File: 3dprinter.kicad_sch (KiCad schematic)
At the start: 35 parts, among them J1 6P IDC CONNECTOR, J17 Conn_01x02, J2 USB_B, SW1 SW_Push, U1 ATmega2560-16A, U2 CH340G, U3 LM78M05_TO252, Y1 16MHZ, Y2 12MHZ

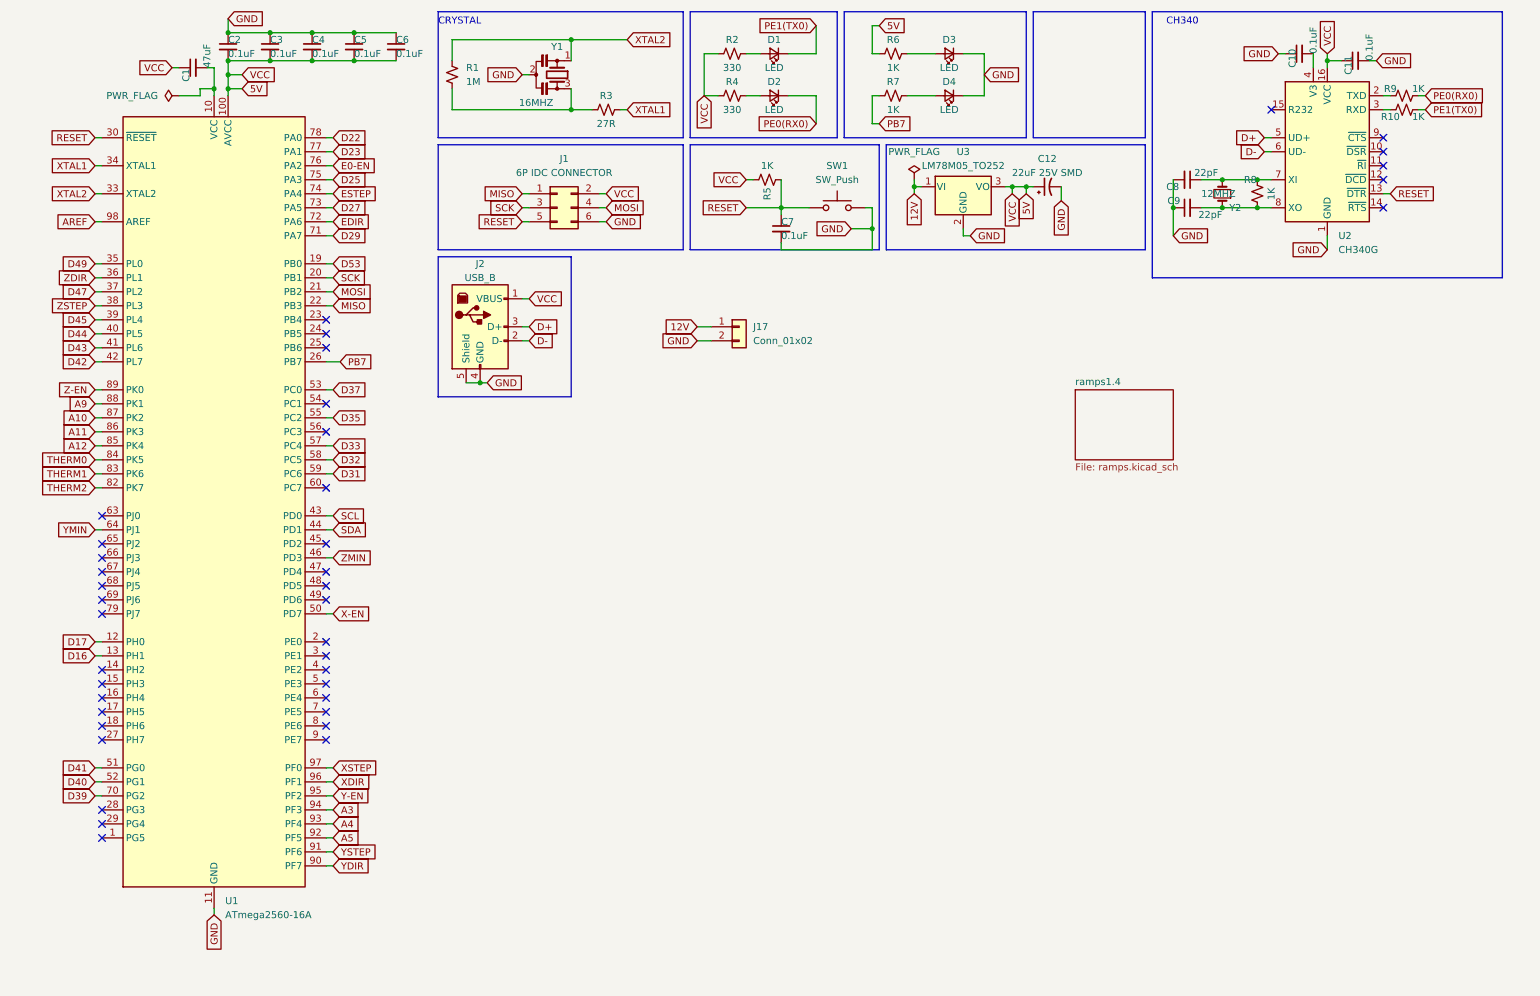
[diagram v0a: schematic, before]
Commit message: Schematic_ok
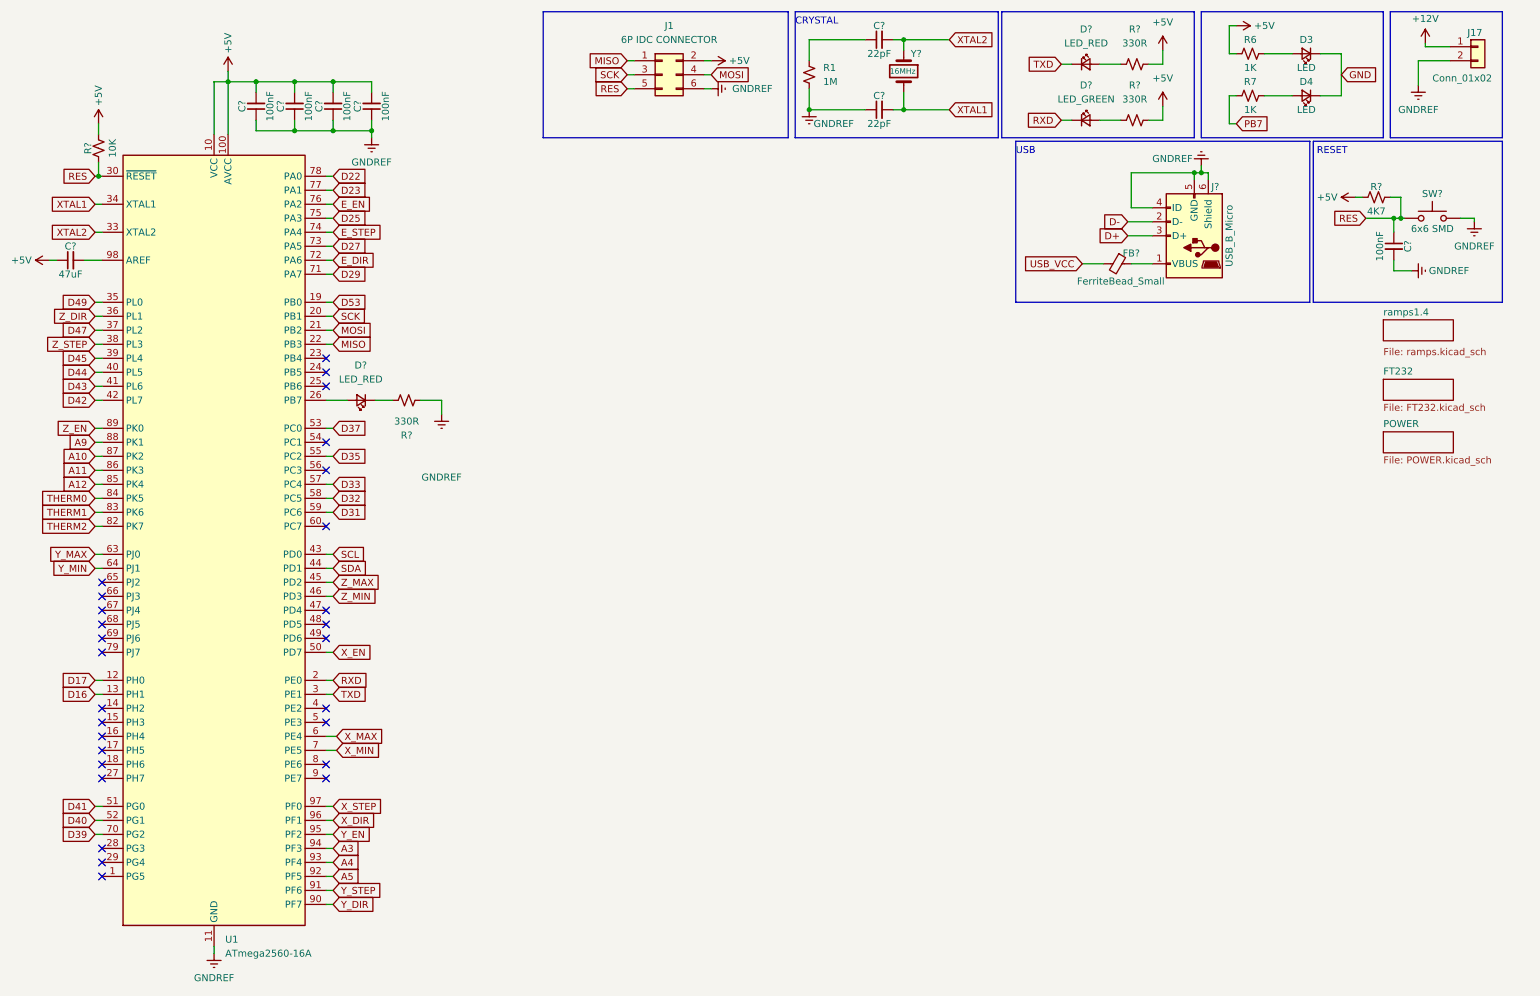
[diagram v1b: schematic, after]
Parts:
- removed C1: 47uF, Capacitor_SMD:C_0805_2012Metric, symbol Device:C_Small
- removed C10, C11, C2, C3, C4, C5, C6, C7: 0.1uF, Capacitor_SMD:C_0805_2012Metric, symbol Device:C_Small
- removed C12: 22uF 25V SMD, Capacitor_SMD:CP_Elec_6.3x7.7, symbol Device:C_Polarized_Small_US
- removed C8, C9: 22pF, Capacitor_SMD:C_0805_2012Metric, symbol Device:C_Small
- removed D1, D2: LED, LED_SMD:LED_0805_2012Metric, symbol Device:LED_Small
- removed J2: USB_B, Connector_USB:USB_B_Lumberg_2411_02_Horizontal, symbol Connector:USB_B
- removed R10, R8, R9: 1K, Resistor_SMD:R_0805_2012Metric, symbol Device:R_Small_US
- removed R2, R4: 330, Resistor_SMD:R_0805_2012Metric, symbol Device:R_Small_US
- removed R3: 27R, Resistor_SMD:R_0805_2012Metric, symbol Device:R_Small_US
- removed R5: 1K, Resistor_SMD:R_0805_2012Metric_Pad1.20x1.40mm_HandSolder, symbol Device:R_Small_US
- removed SW1: SW_Push, Button_Switch_SMD:SW_Push_1P1T_NO_6x6mm_H9.5mm, symbol Switch:SW_Push
- removed U2: CH340G, Package_SO:SOIC-16_3.9x9.9mm_P1.27mm, symbol Interface_USB:CH340G
- removed U3: LM78M05_TO252, Package_TO_SOT_SMD:TO-252-2, symbol Regulator_Linear:LM78M05_TO252
- removed Y1: 16MHZ, Crystal:Crystal_SMD_HC49-SD, symbol Device:Resonator_Small
- removed Y2: 12MHZ, Crystal:Crystal_SMD_HC49-SD, symbol Device:Crystal_Small
- added C?: 47uF, Capacitor_SMD:C_0805_2012Metric_Pad1.18x1.45mm_HandSolder, symbol Device:C_Small
- added C? (x4): 100nF, Capacitor_SMD:C_0805_2012Metric_Pad1.18x1.45mm_HandSolder, symbol Device:C_Small
- added C?: 100nF, Capacitor_SMD:C_0805_2012Metric, symbol Device:C_Small
- added C? (x2): 22pF, Capacitor_SMD:C_0805_2012Metric_Pad1.18x1.45mm_HandSolder, symbol Device:C_Small
- added D? (x2): LED_RED, LED_SMD:LED_0805_2012Metric_Pad1.15x1.40mm_HandSolder, symbol Device:LED_Small
- added D?: LED_GREEN, LED_SMD:LED_0805_2012Metric_Pad1.15x1.40mm_HandSolder, symbol Device:LED_Small
- added FB?: FerriteBead_Small, Capacitor_SMD:C_1206_3216Metric, symbol Device:FerriteBead_Small
- added J?: USB_B_Micro, Connector_USB:USB_Micro-B_GCT_USB3076-30-A, symbol Connector:USB_B_Micro
- added R?: 10K, Resistor_SMD:R_0805_2012Metric_Pad1.20x1.40mm_HandSolder, symbol Device:R_Small_US
- added R? (x3): 330R, Resistor_SMD:R_0805_2012Metric_Pad1.20x1.40mm_HandSolder, symbol Device:R_Small_US
- added R?: 4K7, Resistor_SMD:R_0805_2012Metric, symbol Device:R_Small_US
- added SW?: 6x6 SMD, Button_Switch_SMD:SW_Push_1P1T_NO_6x6mm_H9.5mm, symbol Switch:SW_Push
- added Y?: 16MHz, Crystal:Crystal_SMD_HC49-SD, symbol Device:Crystal
- J1: footprint Connector_PinHeader_2.54mm:PinHeader_2x03_P2.54mm_Vertical -> Connector_PinHeader_1.00mm:PinHeader_2x03_P1.00mm_Vertical
- J17: footprint TerminalBlock_Phoenix:TerminalBlock_Phoenix_MKDS-1,5-2-5.08_1x02_P5.08mm_Horizontal -> Connector_Phoenix_MSTB:PhoenixContact_MSTBVA_2,5_2-G-5,08_1x02_P5.08mm_Vertical
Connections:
- net 5V is gone; now on net +5V: J1.2 (Pin_2), R6.1, U1.100 (AVCC)
- net D+: now also J?.3 (D+)
- net D-: now also J?.2 (D-)
- net GND: no longer J1.6 (Pin_6), J17.2 (Pin_2), U1.11 (GND), U1.32 (GND), U1.62 (GND), U1.81 (GND), U1.99 (GND)
- net PB7: no longer U1.26 (PB7)
- net XTAL1: now also C?.2, Y?.2
- net XTAL2: now also C?.2, Y?.1; no longer R1.1
- net GNDREF: now reaches R1.2
- net GNDREF: now also J1.6 (Pin_6), J17.2 (Pin_2), U1.11 (GND), U1.32 (GND), U1.62 (GND), U1.81 (GND), U1.99 (GND), C?.1, C?.1, C?.1, C?.1, C?.1, C?.2, J?.4 (ID), J?.5 (GND), J?.6 (Shield), R?.1, SW?.2
- net +5V: now reaches U1.10 (VCC), U1.31 (VCC), U1.61 (VCC), U1.80 (VCC)
- net +5V: now also C?.1, C?.2, C?.2, C?.2, C?.2, R?.1, R?.2, R?.2, R?.2
- net RXD: now reaches U1.2 (PE0)
- net RXD: now also D?.1 (K)
- net TXD: now reaches U1.3 (PE1)
- net TXD: now also D?.1 (K)
- net Z_MAX: now reaches U1.45 (PD2)
- net X_MAX: now reaches U1.6 (PE4)
- net Y_MAX: now reaches U1.63 (PJ0)
- net X_MIN: now reaches U1.7 (PE5)
- net 12V renamed +12V
- net AREF: no longer names the net of U1.98 (AREF)
- net AREF: now also C?.2
- net E0-EN renamed E_EN
- net EDIR renamed E_DIR
- net ESTEP renamed E_STEP
- net RESET renamed RES
- net RES: now also C?.1, R?.1, R?.2, SW?.1
- net X-EN renamed X_EN
- net XDIR renamed X_DIR
- net XSTEP renamed X_STEP
- net Y-EN renamed Y_EN
- net YDIR renamed Y_DIR
- net YMIN renamed Y_MIN
- net YSTEP renamed Y_STEP
- net Z-EN renamed Z_EN
- net ZDIR renamed Z_DIR
- net ZMIN renamed Z_MIN
- net ZSTEP renamed Z_STEP
- new net: D?.2 (A), R?.1 (x2)
- new net: C?.1, R1.1
- new net: D?.2 (A), U1.26 (PB7)
- new net: D?.1 (K), R?.2
- new net: FB?.1, J?.1 (VBUS)
- new net USB_VCC: FB?.2
- no-connect marks 40 -> 28
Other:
- added sheet FT232 (FT232.kicad_sch)
- added sheet POWER (POWER.kicad_sch)
- note added: "RESET"
- note added: "USB"
- note removed: "CH340"
- moved on the sheet: D3, D4, J1, J17, R1, R6, R7, U1
